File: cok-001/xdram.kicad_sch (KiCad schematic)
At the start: 74 parts, among them Q1201 RK7002, Q1202 SST2222AT, Q1301 RK7002, Q1302 SST2222AT, U1201 Y0_XDR0, U1202 Y0_XDR1, U1301 Y1_XDR0, U1302 Y1_XDR1

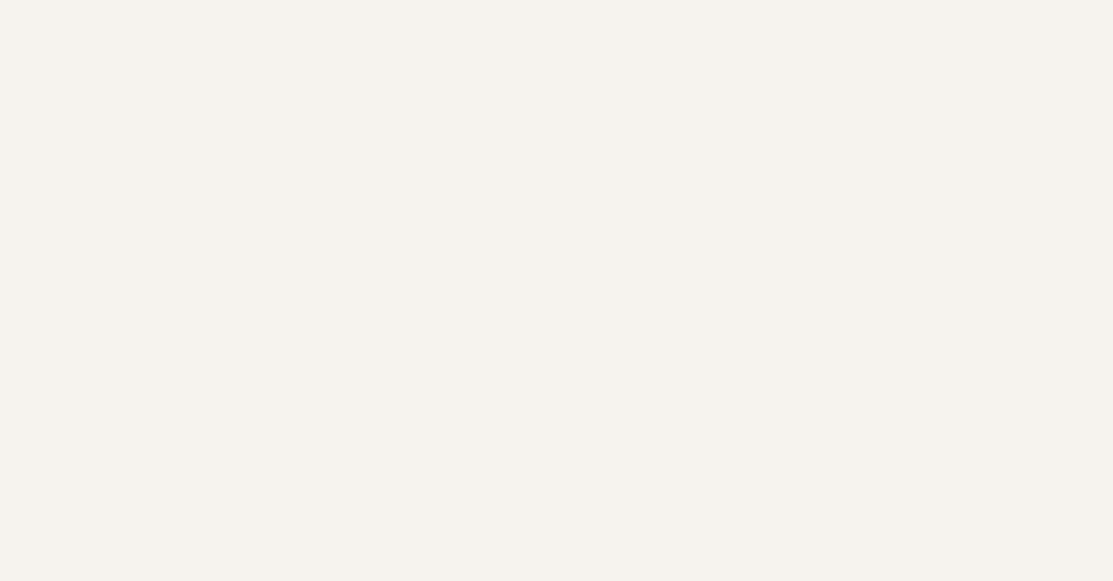
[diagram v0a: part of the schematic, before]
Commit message: ram lines
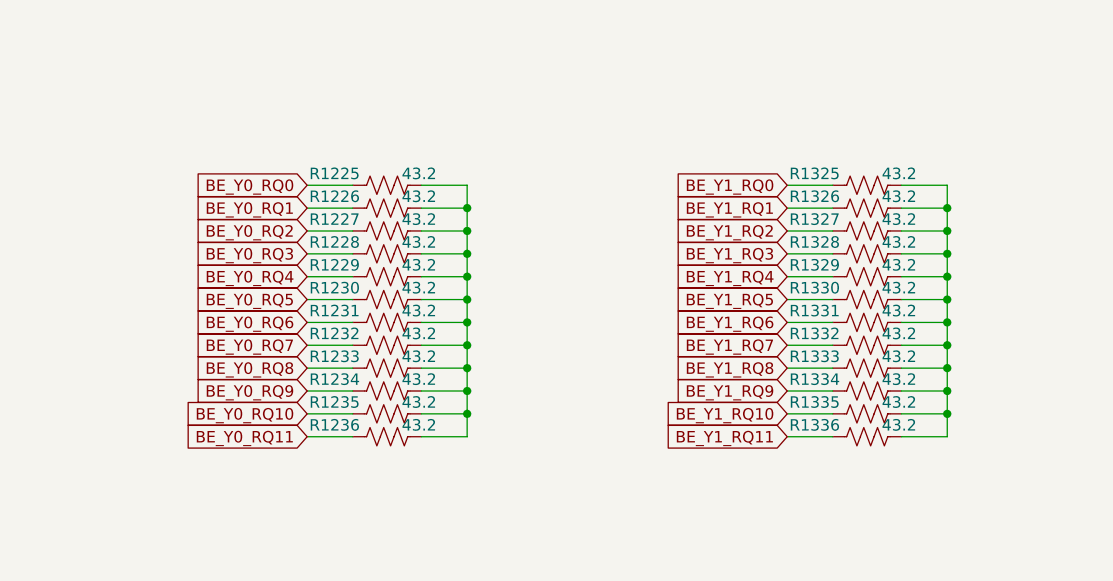
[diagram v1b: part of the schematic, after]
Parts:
- added R1225, R1226, R1227, R1228, R1229, R1230, R1231, R1232, R1233, R1234, R1235, R1236, R1325, R1326, R1327, R1328, R1329, R1330, R1331, R1332, R1333, R1334, R1335, R1336: 43.2, Resistor_SMD:R_0402_1005Metric, symbol Device:R_US
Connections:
- net BE_Y0_RQ0: now also R1225.1
- net BE_Y0_RQ1: now also R1226.1
- net BE_Y0_RQ10: now also R1235.1
- net BE_Y0_RQ11: now also R1236.1
- net BE_Y0_RQ2: now also R1227.1
- net BE_Y0_RQ3: now also R1228.1
- net BE_Y0_RQ4: now also R1229.1
- net BE_Y0_RQ5: now also R1230.1
- net BE_Y0_RQ6: now also R1231.1
- net BE_Y0_RQ7: now also R1232.1
- net BE_Y0_RQ8: now also R1233.1
- net BE_Y0_RQ9: now also R1234.1
- net BE_Y1_RQ0: now also R1325.1
- net BE_Y1_RQ1: now also R1326.1
- net BE_Y1_RQ10: now also R1335.1
- net BE_Y1_RQ11: now also R1336.1
- net BE_Y1_RQ2: now also R1327.1
- net BE_Y1_RQ3: now also R1328.1
- net BE_Y1_RQ4: now also R1329.1
- net BE_Y1_RQ5: now also R1330.1
- net BE_Y1_RQ6: now also R1331.1
- net BE_Y1_RQ7: now also R1332.1
- net BE_Y1_RQ8: now also R1333.1
- net BE_Y1_RQ9: now also R1334.1
- new net: R1325.2, R1326.2, R1327.2, R1328.2, R1329.2, R1330.2, R1331.2, R1332.2, R1333.2, R1334.2, R1335.2, R1336.2
- new net: R1225.2, R1226.2, R1227.2, R1228.2, R1229.2, R1230.2, R1231.2, R1232.2, R1233.2, R1234.2, R1235.2, R1236.2
